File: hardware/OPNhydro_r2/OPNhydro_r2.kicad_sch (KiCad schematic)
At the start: 161 parts, among them J1 MKDS, J2 MKDS, J3 BNC, J4 BNC, J5 BNC, M1 ESP32-C6-DEVKIT, M2 ATLAS_EZO_pH, M3 ATLAS_EZO_EC, M4 ATLAS_EZO_RTD, P1 MSTB_0.2", P10 ANKO_A200SX, P11 ANKO_A200SX, P12 ANKO_A200SX, P2 PHR-4, P3 MC_0.2", P4 DC40F-2460, P5 PHR-4, P6 MC_0.15", P7 XH_2.5mm, P8 XH_2.5mm, P9 XH_2.5mm, SW1 FLOAT, SW2 FLOAT, T1 AON6407, T2 BT3904, T3 IRLR2905, T4 BT3904, T5 AO3400A, U1 TPS62933, U2 AZ1117-3.3, U3 ADM3260, U4 ADM3260, U5 TMC2209, U6 TMC2209, U7 TMC2209

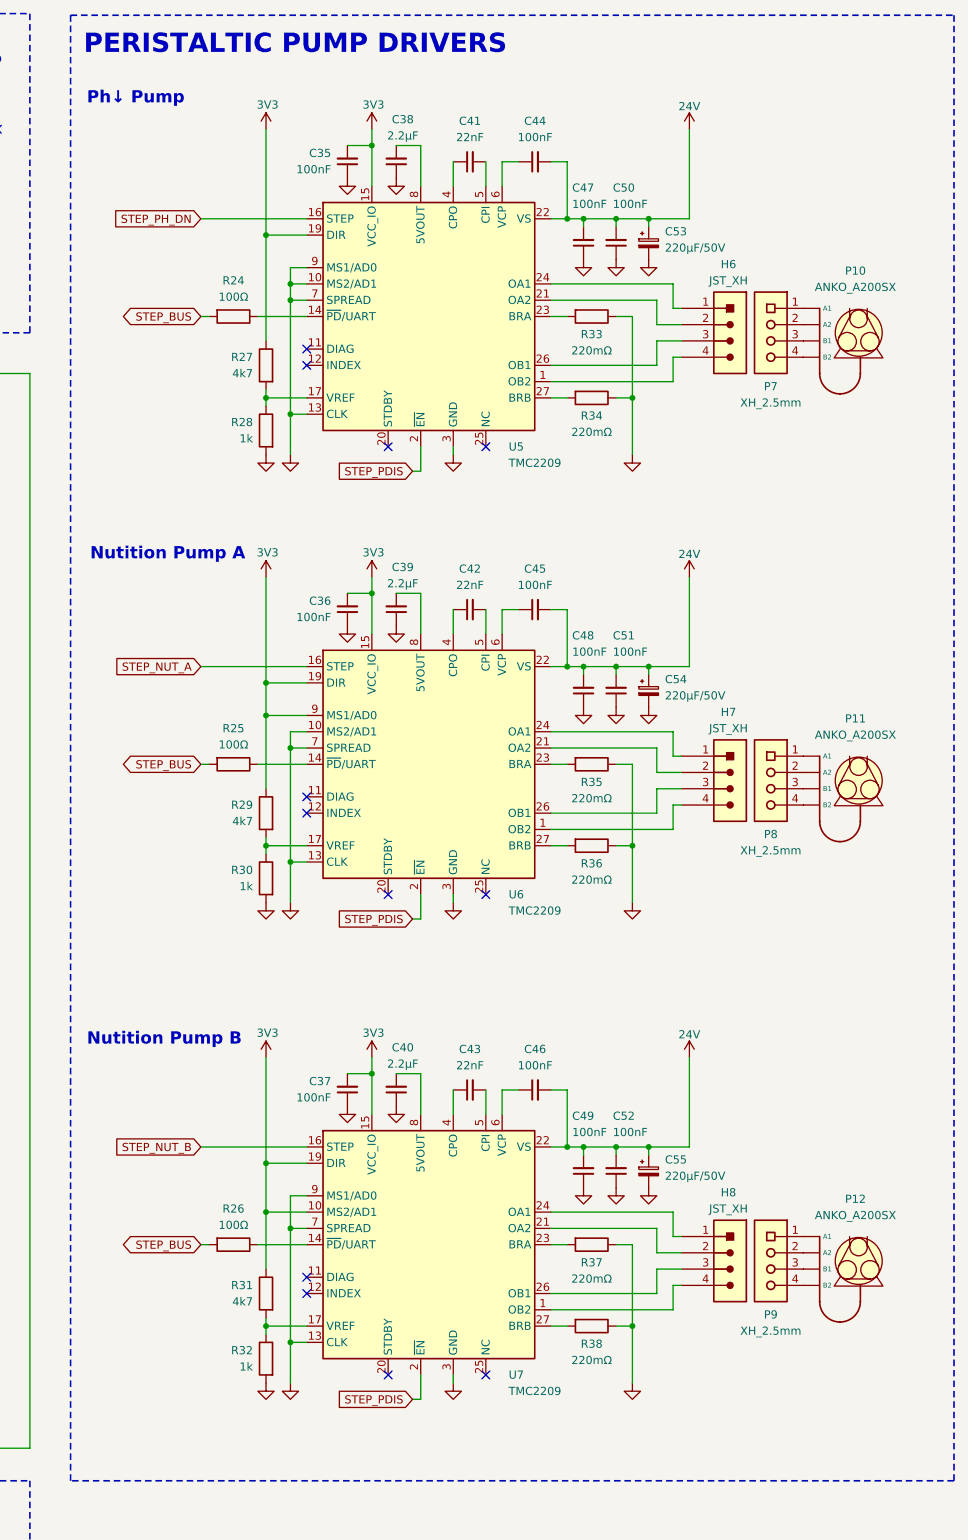
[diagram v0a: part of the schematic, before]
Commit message: update
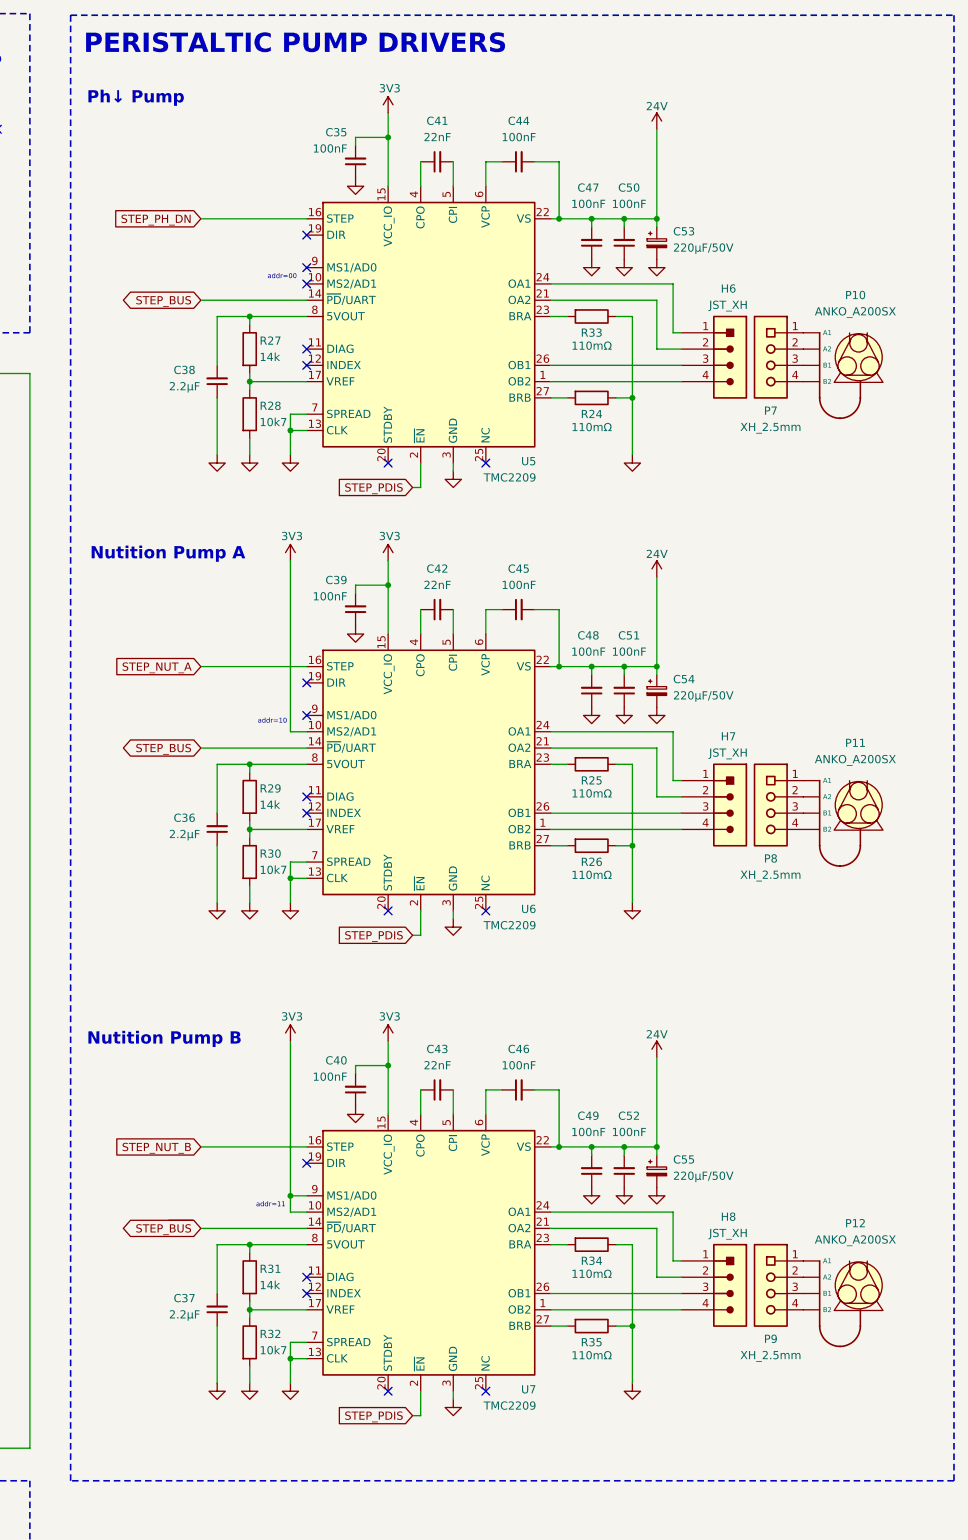
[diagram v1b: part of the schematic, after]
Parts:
- removed C36, C37: 100nF, Coert-Vonk:CAP X7R 100nF ±10 50V 0402 Murata, symbol Coert-Vonk:CAP X7R 100nF ±10% 50V 0402 Murata
- removed C39, C40: 2.2μF, Coert-Vonk:CAP X7R 2.2μF ±10 10V 0603 Murata, symbol Coert-Vonk:CAP X7R 2.2μF ±10% 10V 0603 Murata
- removed R24, R25, R26: 100Ω, Coert-Vonk:RES 100Ω ±1 18W Yageo 0805, symbol Coert-Vonk:RES 100Ω ±1% 1/8W 0805 Yageo
- removed R27, R29, R31: 4k7, Coert-Vonk:RES 0805 YAGEO, symbol Coert-Vonk:RES 4.7kΩ ±1% 1/8W 0805 Yageo
- removed R28, R30, R32: 1k, Coert-Vonk:RES 0805 YAGEO, symbol Coert-Vonk:RES 1kΩ ±1% 1/8W 0805 Yageo
- removed R34, R35, R36, R37, R38: 220mΩ, Coert-Vonk:RES 0805 YAGEO, symbol Coert-Vonk:RES 220mΩ ±1% 1/4W 0805 Yageo
- added C36, C37: 2.2μF, Coert-Vonk:CAP X7R 2.2μF ±10 10V 0603 Murata, symbol Coert-Vonk:CAP X7R 2.2μF ±10% 10V 0603 Murata
- added C39, C40: 100nF, Coert-Vonk:CAP X7R 100nF ±10 50V 0402 Murata, symbol Coert-Vonk:CAP X7R 100nF ±10% 50V 0402 Murata
- added R24, R25, R26, R34, R35: 110mΩ, Coert-Vonk:RES 0805 YAGEO, symbol Coert-Vonk:RES 110mΩ ±1% 1/8W 0805 Susumu
- added R27, R29, R31: 14k, Coert-Vonk:RES 0805 YAGEO, symbol Coert-Vonk:RES 14kΩ ±1% 1/8W 0805 Yageo
- added R28, R30, R32: 10k7, Coert-Vonk:RES 0805 YAGEO, symbol Coert-Vonk:RES 10.7kΩ ±1% 1/8W 0805 Yageo
- R33: value 220mΩ -> 110mΩ; symbol Coert-Vonk:RES 220mΩ ±1% 1/4W 0805 Yageo -> Coert-Vonk:RES 110mΩ ±1% 1/8W 0805 Susumu; DKPN 311-0.22LUCT-ND -> RL12S.11FCT-ND
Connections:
- net 3V3: now also U6.10 (MS2/AD1), U7.9 (MS1/AD0), C39.2, C40.2; no longer U5.19 (DIR), U6.19 (DIR), U6.9 (MS1/AD0), U7.19 (DIR)
- net GND: now also C36.1, C37.1, C39.1, C40.1, R24.2, R25.2, R26.2, R28.1, R30.1, R32.1, R34.2, R35.2; no longer U5.10 (MS2/AD1), U5.9 (MS1/AD0), U6.10 (MS2/AD1), U7.9 (MS1/AD0)
- net STEP_BUS: now also U5.14 (~{PD}/UART), U6.14 (~{PD}/UART), U7.14 (~{PD}/UART)
- net at C38.2, U5.8 (5VOUT): now also R27.2
- net at U7.23 (BRA): now also R34.1
- net at U6.17 (VREF): now also R29.1, R30.2
- net at U7.17 (VREF): now also R31.1, R32.2
- net at U7.27 (BRB): now also R35.1
- net at U7.8 (5VOUT): now also C37.2, R31.2
- net at U5.17 (VREF): now also R27.1, R28.2
- net at U5.27 (BRB): now also R24.1
- net at U6.27 (BRB): now also R26.1
- net at U6.23 (BRA): now also R25.1
- net at U6.8 (5VOUT): now also C36.2, R29.2
- no-connect marks 25 -> 31
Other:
- note added: "addr=00"
- note added: "addr=10"
- note added: "addr=11"
- moved on the sheet: C35, C38, C41, C44, C47, C50, C53, H6, H7, P10, P11, P12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

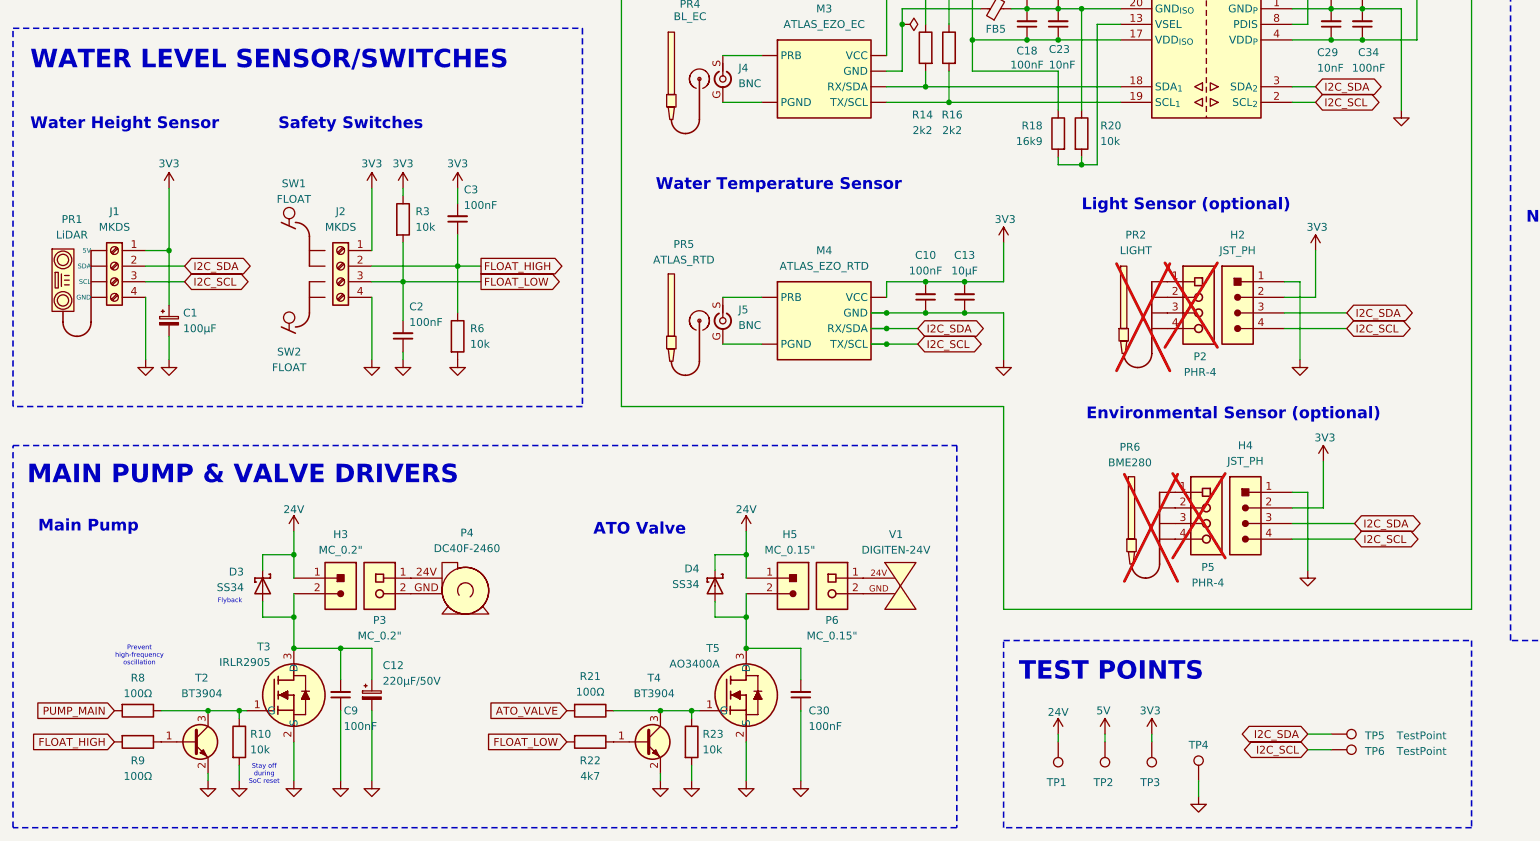
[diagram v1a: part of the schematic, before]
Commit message: update
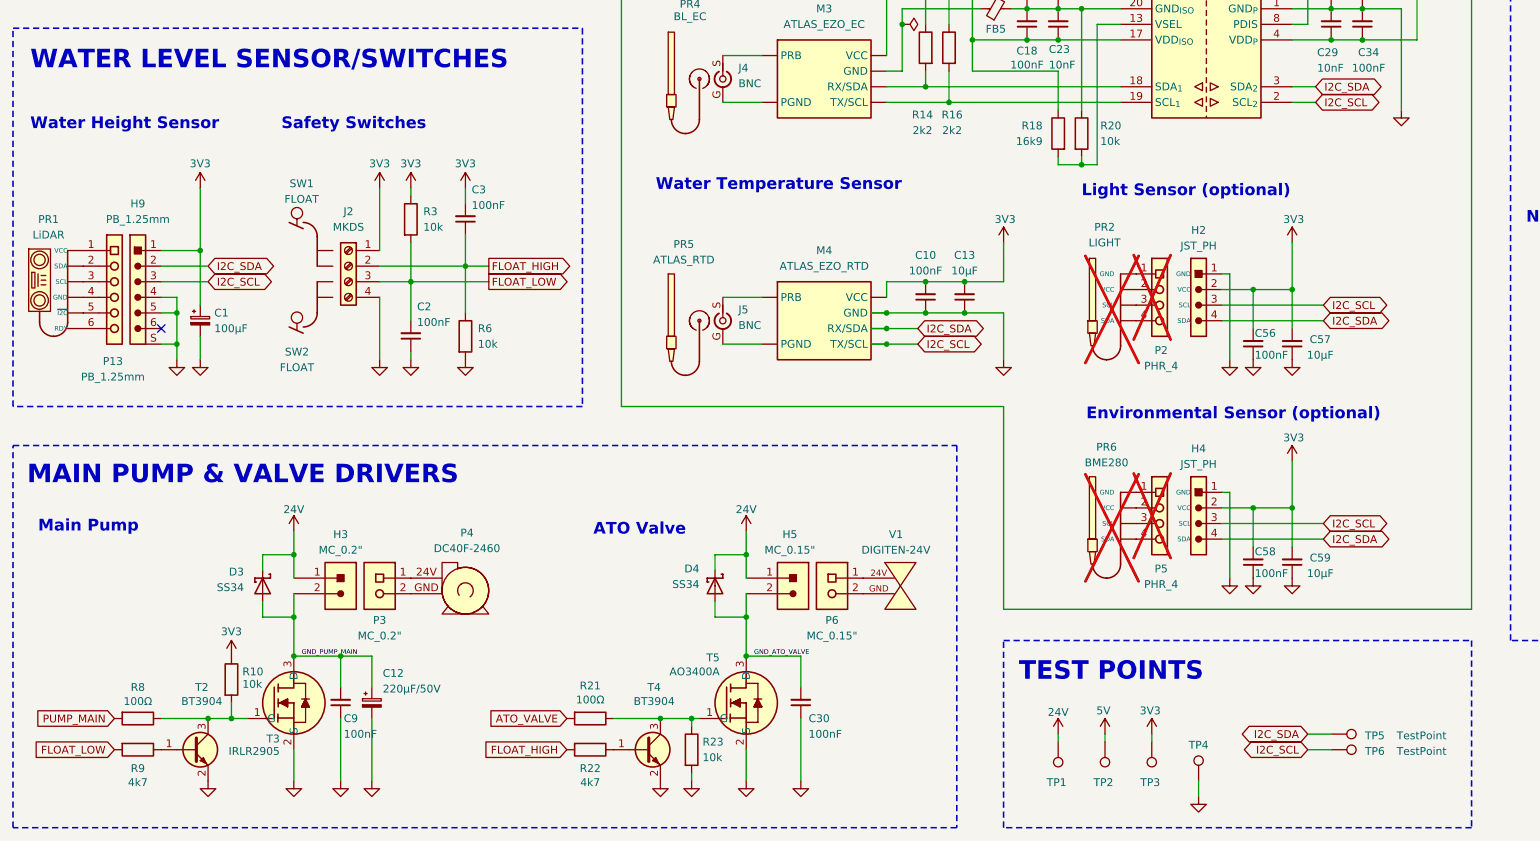
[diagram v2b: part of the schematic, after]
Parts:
- removed J1: MKDS, Coert-Vonk:TERM BLK 4POS SCREW 3.5mm, symbol Coert-Vonk:TERM BLK SCREW 4POS MKDS 3.5mm
- removed PR2: LIGHT, symbol Coert-Vonk:PROBE_LIGHT
- removed R9: 100Ω, Coert-Vonk:RES 100Ω ±1 18W Yageo 0805, symbol Coert-Vonk:RES 100Ω ±1% 1/8W 0805 Yageo
- added C56, C58: 100nF, Coert-Vonk:CAP X7R 100nF ±10 50V 0402 Murata, symbol Coert-Vonk:CAP X7R 100nF ±10% 50V 0402 Murata
- added C57, C59: 10μF, Coert-Vonk:CAP X5R 10μF ±10 16V 0805 Murata GRM, symbol Coert-Vonk:CAP X5R 10μF ±10% 16V 0805 Murata GRM
- added H9: PB_1.25mm, Coert-Vonk:TERM BLK HDR 6POS PB 1.25mm Molex, symbol Coert-Vonk:TERM BLK HDR 6POS MOLEX-PB 1.25mm
- added P13: PB_1.25mm, Coert-Vonk:TERM BLK PLG 6POS MOLEX-PB 1.25mm, symbol Coert-Vonk:TERM BLK PLG 6POS MOLEX-PB 1.25mm
- added PR2: LIGHT, symbol Coert-Vonk:PROBE LIGHT
- added R9: 4k7, Coert-Vonk:RES 0805 YAGEO, symbol Coert-Vonk:RES 4.7kΩ ±1% 1/8W 0805 Yageo
- H1: MFR (none) -> Phoenix Connect; MPN (none) -> 1757242
- H2, H4: MFR (none) -> JST; PN (none) -> S4B-PH-K-S
- H3: MFR (none) -> Phoenix Connect; MPN (none) -> 1836189
- H5: MFR (none) -> Phoenix Connect; MPN (none) -> 1803277
- J2: MFR (none) -> Phoenix Contact; MPN (none) -> 1751264
- P1: MFR (none) -> Phoenix Connect; MPN (none) -> 1757019
- P2, P5: value PHR-4 -> PHR_4
- P3: MFR (none) -> Phoenix Connect; MPN (none) -> 1836079
- P6: MFR (none) -> Phoenix Connect; MPN (none) -> 1803578
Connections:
- net 3V3: now also R10.2, C56.2, C57.2, C58.2, C59.2, H9.1
- net FLOAT_HIGH: now also R22.1
- net FLOAT_LOW: now also R9.1; no longer R22.1
- net GND: now also C56.1, C57.1, C58.1, C59.1, H9.4, H9.5, H9.S, H9.S2; no longer R10.1
- net I2C_SCL: now also H2.3 (SCL), H4.3 (SCL), H9.3; no longer H2.4 (I2C_SCL), H4.4 (I2C_SCL)
- net I2C_SDA: now also H2.4 (SDA), H4.4 (SDA), H9.2; no longer H2.3 (I2C_SDA), H4.3 (I2C_SDA)
- net GND_PUMP_MAIN: now reaches C12.1, C9.2, D3.A, H3.2, T3.3 (D)
- net at P2.1: now also PR2.1 (GND)
- net at P2.2: now also PR2.2 (VCC)
- net at P2.3: now also PR2.3 (SCL)
- net at P2.4: now also PR2.4 (SDA)
- net GND_ATO_VALVE: now reaches C30.2, D4.A, H5.2, T5.3 (D)
- net at R8.2, T2.3 (C), T3.1 (G): now also R10.1; no longer R10.2
- net at PR1.1 (VCC): now also P13.1
- net at PR1.2 (SDA): now also P13.2
- net at PR1.3 (SCL): now also P13.3
- net at PR1.4 (RDY): now also P13.6
- net at T2.1 (B): now also R9.2
- new net: P13.4, PR1.4 (RDY)
- new net: P13.5, PR1.4 (RDY)
- no-connect marks 31 -> 32
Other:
- note removed: "Flyback"
- note removed: "Prevent high-frequency oscillation"
- note removed: "Stay off during SoC reset"
- moved on the sheet: C1, C12, C2, C3, C30, C9, J2, P2, P5, R10, R21, R22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
